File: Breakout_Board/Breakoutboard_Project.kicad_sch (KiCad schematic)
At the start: 17 parts, among them J1 Conn_01x17, J2 Conn_01x17, J3 Conn_02x06_Top_Bottom, J4 Conn_01x04, U2 STM32F411

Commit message: preliminary
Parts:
- J1, J2: footprint Package_QFP:LQFP-176_24x24mm_P0.5mm -> Connector_PinHeader_2.54mm:PinHeader_1x17_P2.54mm_Vertical
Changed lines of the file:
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@@
 	)
 	(image
-		(at -96.52 87.63)
+		(at -130.175 94.615)
 		(scale 2.05924)
 		(data "iVBORw0KGgoAAAANSUhEUgAABLoAAANjCAYAAACtDnMJAAAABHNCSVQICAgIfAhkiAAAIABJREFU"
@@
 			)
 		)
-		(property "Footprint" "Package_QFP:LQFP-176_24x24mm_P0.5mm"
+		(property "Footprint" "Connector_PinHeader_2.54mm:PinHeader_1x17_P2.54mm_Vertical"
 			(at 152.4 139.7 0)
 			(hide yes)
@@
 			)
 		)
-		(property "Footprint" "Package_QFP:LQFP-176_24x24mm_P0.5mm"
+		(property "Footprint" "Connector_PinHeader_2.54mm:PinHeader_1x17_P2.54mm_Vertical"
 			(at 129.54 139.7 0)
 			(hide yes)

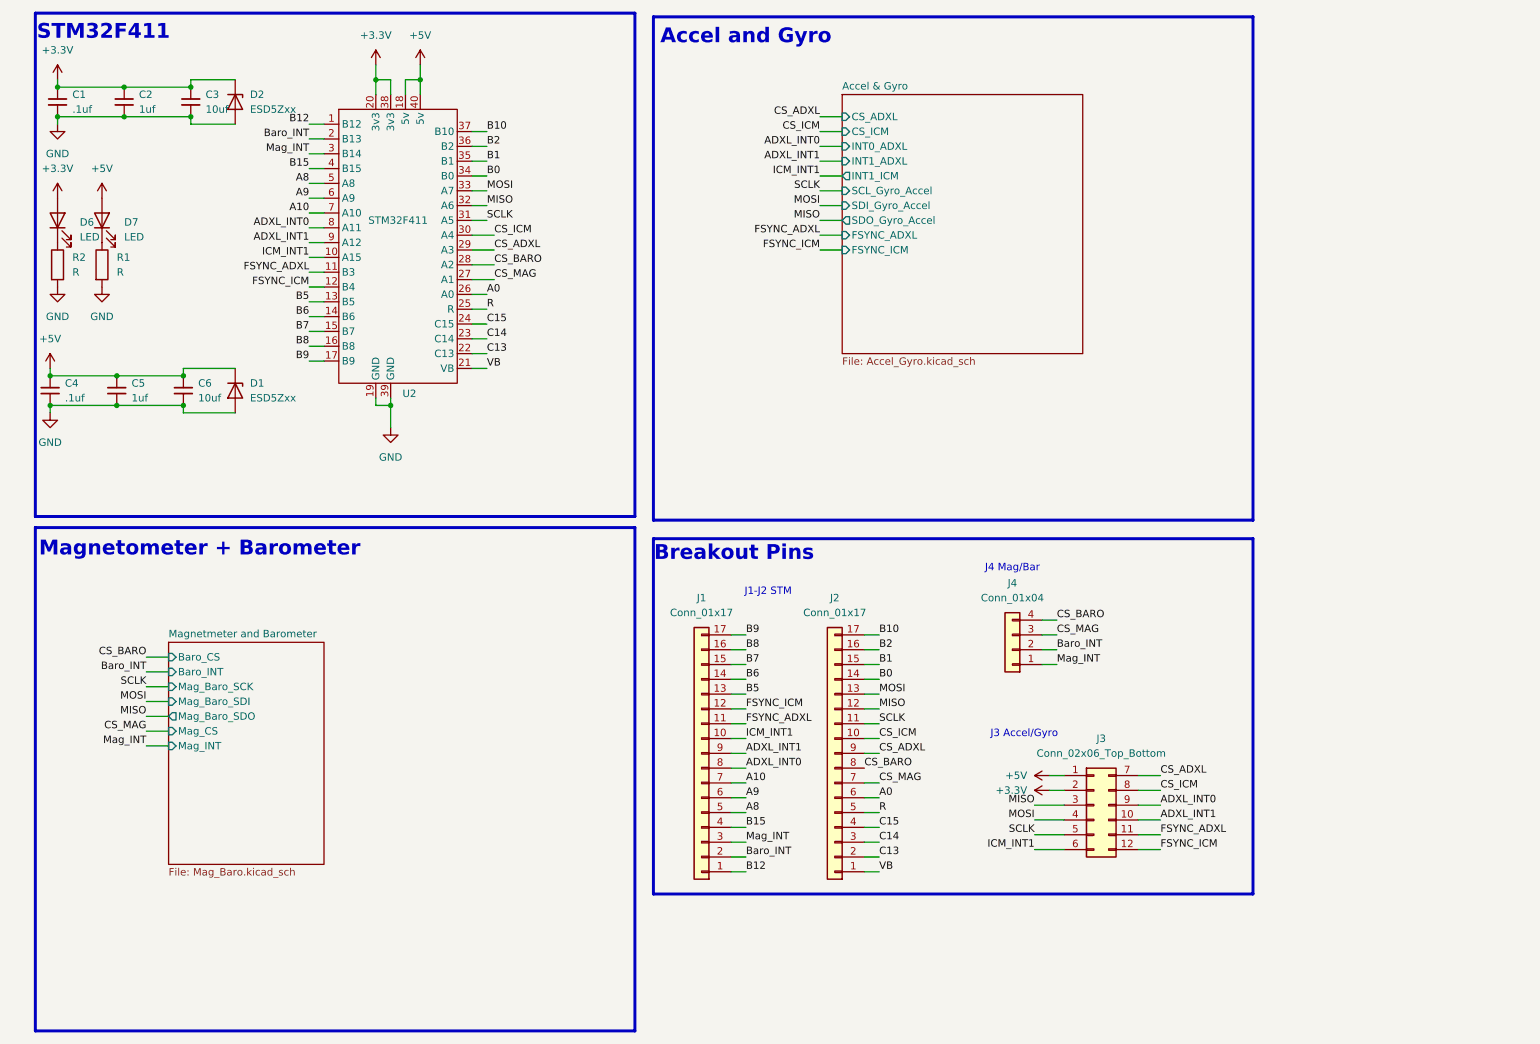
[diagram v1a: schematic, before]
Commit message: ready for routing
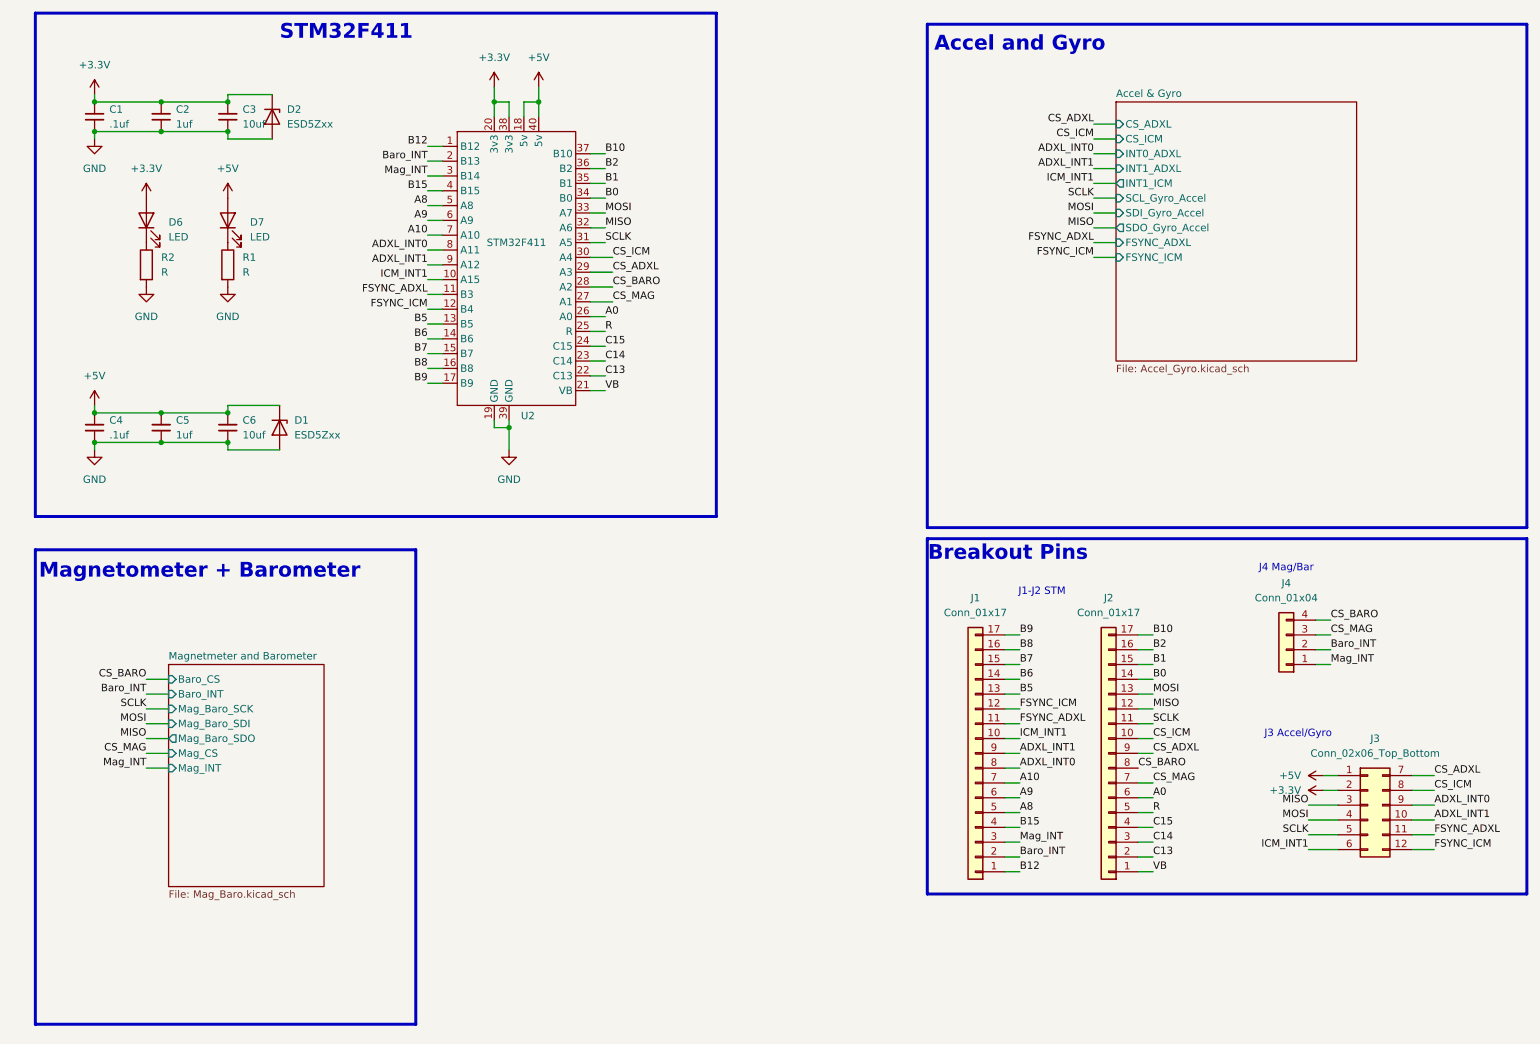
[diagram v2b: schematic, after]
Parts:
- J3: footprint Connector_PinHeader_1.27mm:PinHeader_2x06_P1.27mm_Vertical -> Connector_Hirose:Hirose_DF11-12DP-2DSA_2x06_P2.00mm_Vertical
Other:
- moved on the sheet: C1, C2, C3, C4, C5, C6, D1, D2, D6, D7, J1, J2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
